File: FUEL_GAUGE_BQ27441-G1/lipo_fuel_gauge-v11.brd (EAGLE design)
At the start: 10.2 x 24.1 mm, 11 parts, among them U1 BQ27441-G1

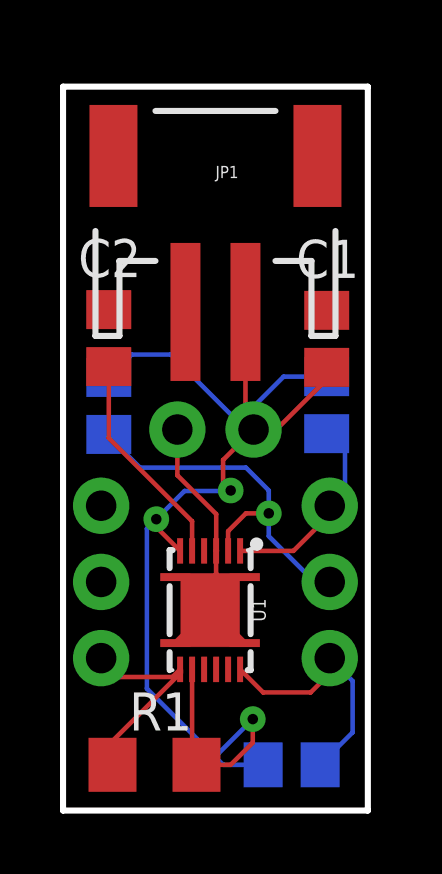
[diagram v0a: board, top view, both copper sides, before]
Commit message: Bin pin pulled down to Vss by 10K resistor
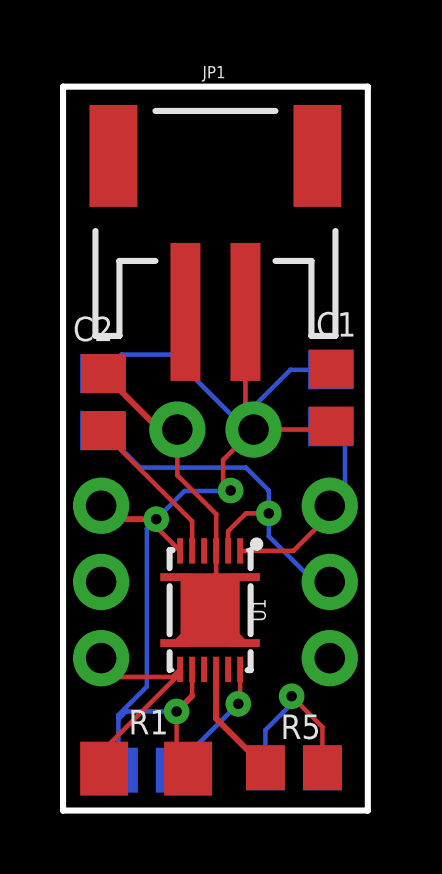
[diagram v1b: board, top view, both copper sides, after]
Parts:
- added R5: 0R, rcl:R0805
- added R6: 10K, rcl:R0805
- moved R4 4.83 mm to (2.79, 1.35)
- moved C2 2.14 mm to (1.35, 13.6)
- moved C1 1.96 mm to (8.94, 13.8)
- moved R1 0.31 mm to (2.77, 1.40)
- moved R2 0.26 mm to (8.92, 13.7)
- moved R3 0.24 mm to (1.32, 13.6)
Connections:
- new net N$1: R5.1, R6.2
- net BIN: now also R5.2
- net GND: now also JP2.3, R6.1
- net GPOUT: no longer JP2.3
- net VCC: now also JP4.1
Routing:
- net N$1: track 0.00 -> 5.56 mm, vias 0 -> 1
- net GPOUT: track 8.40 -> 4.25 mm, vias 0 -> 1
- net BIN: track 0.00 -> 3.96 mm
- net GND: track 10.9 -> 14.2 mm
- net VCC: track 42.9 -> 40.3 mm
- net VDD: track 7.29 -> 5.23 mm
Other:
- board text added: "OUT"
- board text removed: "BIN"
- board text removed: "GPOUT"
